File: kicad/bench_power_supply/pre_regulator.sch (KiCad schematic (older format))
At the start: 29 parts, among them K2 CONN_01X02, Q1 IRF5210PBF, Q2 IRF5210PBF, Q3 MMBT5401, Q4 MMBT5401, Q5 SCR

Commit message: added files from mint
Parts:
- removed K2: CONN_01X02, symbol CONN_01X02
- B1: symbol D_BRIDGE -> D_Bridge
- C1, C2, C3: symbol C_SMALL -> C_Small
- C4: symbol CP1_SMALL -> CP1_Small
- D1, D2, D3: symbol D_SMALL -> D_Small
- R1, R10, R11, R12, R13, R2, R3, R4, R5, R6, R7, R8, R9: symbol R_SMALL -> R_Small
- Z1, Z2: symbol ZENERSMALL -> ZENERsmall
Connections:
- net labels added: AC1, AC2
- wire segments 94 -> 60
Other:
- moved on the sheet: Q1, Q2, Q3, Q4, Q5

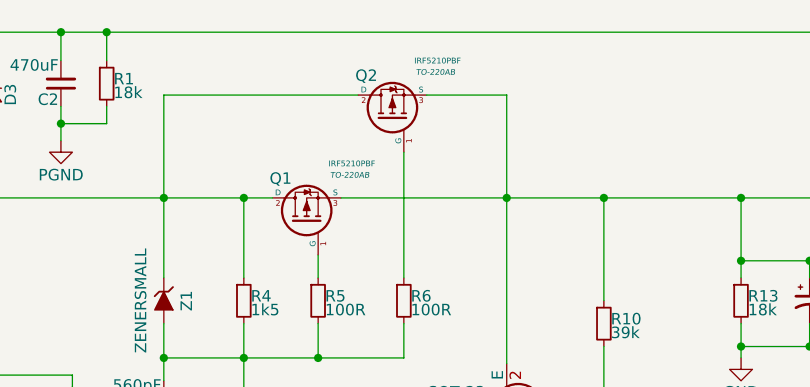
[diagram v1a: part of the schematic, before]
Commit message: commiting before install linux mint
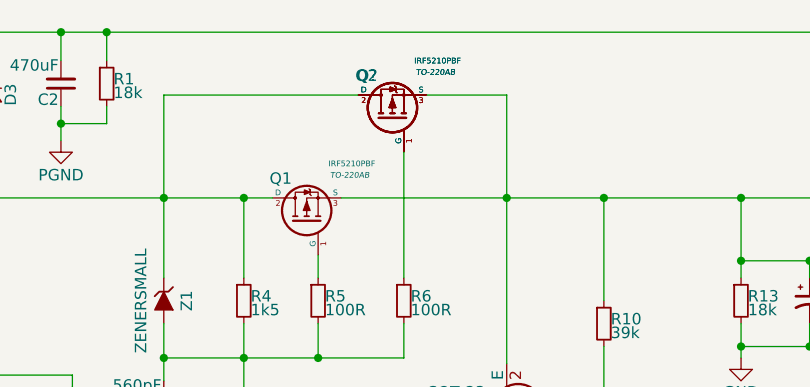
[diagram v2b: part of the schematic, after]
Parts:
- added Q?: IRF5210PBF, TO-220AB, symbol IRF5210PBF
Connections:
- net POut: now also Q?.3 (S)
- net at B1.3 (+), D3.2 (A), Q1.2 (D)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: now also Q?.2 (D)
- net at Q2.1 (G), R6.1: now also Q?.1 (G)
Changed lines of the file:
@@
 Text HLabel 1150 2200 0    60   Input ~ 0
 AC2
+$Comp
+L IRF5210PBF Q?
+U 1 1 579692C0
+P 4975 1575
+F 0 "Q?" V 5160 1640 50  0000 L CNN
+F 1 "IRF5210PBF" V 5225 1275 25  0000 L CNN
+F 2 "TO-220AB" V 5175 1300 25  0000 L CIN
+F 3 "~" H 4975 1575 50  0000 L CNN
+	1    4975 1575
+	0    -1   -1   0
+$EndComp
 $EndSCHEMATC
